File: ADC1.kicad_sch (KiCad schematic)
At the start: 21 parts, among them U8 MCP6004

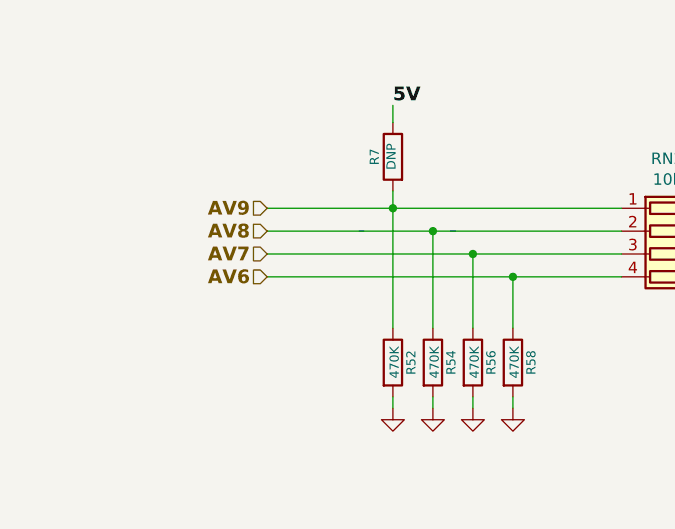
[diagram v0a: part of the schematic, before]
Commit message: haciendo el pcb
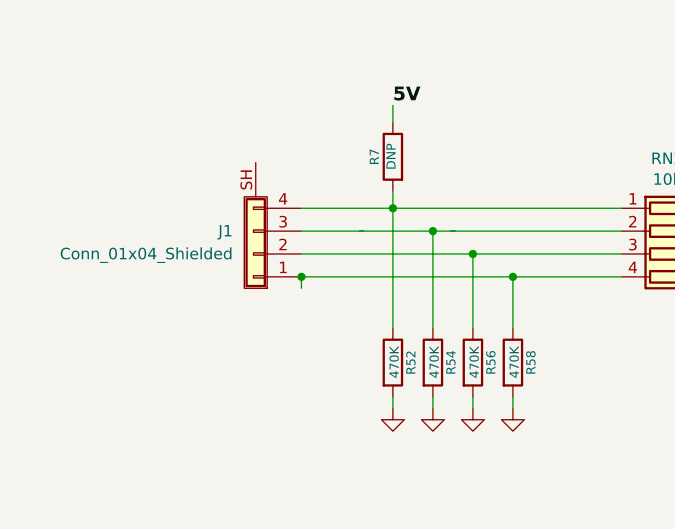
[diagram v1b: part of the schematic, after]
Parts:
- added J1: Conn_01x04_Shielded, Connector_Phoenix_SPT:PhoenixContact_SPT_2.5_4-H-5.0-EX_1x04_P5.0mm_Horizontal, symbol Connector_Generic_Shielded:Conn_01x04_Shielded
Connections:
- net AV6: no longer names the net of R58.1, RN2.4 (R4.1)
- net AV6: now also J1.1 (Pin_1)
- net AV7: no longer names the net of R56.1, RN2.3 (R3.1)
- net AV7: now also J1.2 (Pin_2)
- net AV8: no longer names the net of R54.1, RN2.2 (R2.1)
- net AV8: now also J1.3 (Pin_3)
- net AV9: no longer names the net of R52.1, R7.2, RN2.1 (R1.1)
- net AV9: now also J1.4 (Pin_4)
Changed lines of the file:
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@@
 	)
 	(junction
-		(at 191.77 66.04)
+		(at 87.63 85.09)
 		(diameter 0)
 		(color 0 0 0 0)
 	)
 	(junction
-		(at 87.63 85.09)
+		(at 68.58 87.63)
+		(diameter 0)
+		(color 0 0 0 0)
+	)
+	(junction
+		(at 191.77 66.04)
 		(diameter 0)
 		(color 0 0 0 0)
@@
 	)
 	(junction
-		(at 83.185 82.55)
+		(at 201.93 111.76)
 		(diameter 0)
 		(color 0 0 0 0)
 	)
 	(junction
-		(at 201.93 111.76)
+		(at 78.74 80.01)
 		(diameter 0)
 		(color 0 0 0 0)
 	)
 	(junction
-		(at 78.74 80.01)
+		(at 83.185 82.55)
 		(diameter 0)
 		(color 0 0 0 0)
@@
 	(wire
 		(pts
-			(xy 201.93 130.81) (xy 201.93 132.08)
+			(xy 68.58 85.09) (xy 87.63 85.09)
 		)
 		(stroke
@@
 	(wire
 		(pts
-			(xy 162.56 114.3) (xy 162.56 85.09)
-		)
-		(stroke
-			(width 0)
-			(type default)
-		)
-	)
-	(wire
-		(pts
-			(xy 142.24 109.855) (xy 142.24 80.01)
+			(xy 201.93 130.81) (xy 201.93 132.08)
 		)
 		(stroke
@@
 	(wire
 		(pts
-			(xy 64.77 87.63) (xy 92.075 87.63)
+			(xy 162.56 114.3) (xy 162.56 85.09)
 		)
 		(stroke
@@
 	(wire
 		(pts
-			(xy 83.185 82.55) (xy 104.14 82.55)
+			(xy 142.24 109.855) (xy 142.24 80.01)
 		)
 		(stroke
@@
 	(wire
 		(pts
-			(xy 92.075 87.63) (xy 104.14 87.63)
+			(xy 68.58 87.63) (xy 92.075 87.63)
 		)
 		(stroke
@@
 	(wire
 		(pts
-			(xy 64.77 80.01) (xy 78.74 80.01)
+			(xy 125.73 87.63) (xy 165.1 87.63)
 		)
 		(stroke
@@
 	(wire
 		(pts
-			(xy 87.63 93.345) (xy 87.63 85.09)
+			(xy 83.185 93.345) (xy 83.185 82.55)
 		)
 		(stroke
@@
 	(wire
 		(pts
-			(xy 125.73 87.63) (xy 165.1 87.63)
+			(xy 123.825 85.09) (xy 162.56 85.09)
 		)
 		(stroke
@@
 	(wire
 		(pts
-			(xy 83.185 93.345) (xy 83.185 82.55)
+			(xy 139.065 109.855) (xy 142.24 109.855)
 		)
 		(stroke
@@
 		)
 	)
-	(wire
+	(polyline
 		(pts
-			(xy 123.825 85.09) (xy 162.56 85.09)
+			(xy 74.93 82.55) (xy 75.565 82.55)
 		)
 		(stroke
 			(width 0)
-			(type default)
+			(type dash)
 		)
 	)
 	(wire
 		(pts
-			(xy 139.065 109.855) (xy 142.24 109.855)
+			(xy 78.74 68.58) (xy 78.74 70.485)
 		)
 		(stroke
@@
 		)
 	)
-	(polyline
+	(wire
 		(pts
-			(xy 74.93 82.55) (xy 75.565 82.55)
+			(xy 83.185 82.55) (xy 104.14 82.55)
 		)
 		(stroke
 			(width 0)
-			(type dash)
+			(type default)
 		)
 	)
 	(wire
 		(pts
-			(xy 78.74 68.58) (xy 78.74 70.485)
+			(xy 114.3 85.09) (xy 123.825 85.09)
 		)
 		(stroke
@@
 	(wire
 		(pts
-			(xy 114.3 85.09) (xy 123.825 85.09)
+			(xy 157.48 80.01) (xy 168.91 80.01)
 		)
 		(stroke
@@
 	(wire
 		(pts
-			(xy 157.48 80.01) (xy 168.91 80.01)
+			(xy 127 112.395) (xy 128.905 112.395)
 		)
 		(stroke
@@
 	(wire
 		(pts
-			(xy 127 112.395) (xy 128.905 112.395)
+			(xy 92.075 87.63) (xy 104.14 87.63)
 		)
 		(stroke
@@
 	(wire
 		(pts
+			(xy 68.58 82.55) (xy 83.185 82.55)
+		)
+		(stroke
+			(width 0)
+			(type default)
+		)
+	)
+	(wire
+		(pts
 			(xy 198.12 74.295) (xy 199.39 74.295)
 		)
@@
 	(wire
 		(pts
-			(xy 78.74 93.345) (xy 78.74 80.01)
+			(xy 78.74 80.01) (xy 78.74 93.345)
 		)
 		(stroke
@@
 		)
 	)
-	(wire
+	(polyline
 		(pts
-			(xy 64.77 82.55) (xy 83.185 82.55)
+			(xy 207.01 86.36) (xy 199.39 86.36)
 		)
 		(stroke
 			(width 0)
-			(type default)
+			(type dash)
 		)
 	)
 	(wire
 		(pts
-			(xy 64.77 85.09) (xy 87.63 85.09)
+			(xy 87.63 85.09) (xy 87.63 93.345)
 		)
 		(stroke
@@
 		)
 	)
-	(polyline
+	(wire
 		(pts
-			(xy 207.01 86.36) (xy 199.39 86.36)
+			(xy 217.17 87.63) (xy 219.71 87.63)
 		)
 		(stroke
 			(width 0)
-			(type dash)
+			(type default)
 		)
 	)
 	(wire
 		(pts
-			(xy 217.17 87.63) (xy 219.71 87.63)
+			(xy 144.145 114.935) (xy 144.145 82.55)
 		)
 		(stroke
@@
 	(wire
 		(pts
-			(xy 144.145 114.935) (xy 144.145 82.55)
+			(xy 78.74 80.01) (xy 104.14 80.01)
 		)
 		(stroke
@@
 	(wire
 		(pts
-			(xy 78.74 80.01) (xy 104.14 80.01)
+			(xy 176.53 76.2) (xy 172.72 76.2)
 		)
 		(stroke
@@
 	(wire
 		(pts
-			(xy 176.53 76.2) (xy 172.72 76.2)
+			(xy 68.58 88.9) (xy 68.58 87.63)
 		)
 		(stroke
@@
 	(wire
 		(pts
+			(xy 68.58 80.01) (xy 78.74 80.01)
+		)
+		(stroke
+			(width 0)
+			(type default)
+		)
+	)
+	(wire
+		(pts
 			(xy 191.77 104.14) (xy 198.12 104.14)
 		)
@@
 		)
 	)
-	(hierarchical_label "AV8"
-		(shape input)
-		(at 64.77 82.55 180)
-		(effects
-			(font
-				(size 1.524 1.524)
-				(thickness 0.3048)
-				(bold yes)
-			)
-			(justify right)
-		)
-	)
-	(hierarchical_label "AV6"
-		(shape input)
-		(at 64.77 87.63 180)
-		(effects
-			(font
-				(size 1.524 1.524)
-				(thickness 0.3048)
-				(bold yes)
-			)
-			(justify right)
-		)
-	)
 	(hierarchical_label "AV6_MCU"
 		(shape input)
@@
 		)
 	)
-	(hierarchical_label "AV9"
-		(shape input)
-		(at 64.77 80.01 180)
-		(effects
-			(font
-				(size 1.524 1.524)
-				(thickness 0.3048)
-				(bold yes)
-			)
-			(justify right)
-		)
-	)
 	(hierarchical_label "AV8_MCU"
 		(shape input)
@@
 		)
 	)
-	(hierarchical_label "AV7"
-		(shape input)
-		(at 64.77 85.09 180)
-		(effects
-			(font
-				(size 1.524 1.524)
-				(thickness 0.3048)
-				(bold yes)
-			)
-			(justify right)
-		)
-	)
 	(symbol
 		(lib_id "Device:C")
@@
 					(unit 1)
 				)
+			)
+		)
+	)
+	(symbol
+		(lib_id "Connector_Generic_Shielded:Conn_01x04_Shielded")
+		(at 63.5 85.09 180)
+		(unit 1)
+		(body_style 1)
+		(exclude_from_sim no)
+		(in_bom yes)
+		(on_board yes)
+		(in_pos_files yes)
+		(dnp no)
+		(fields_autoplaced yes)
+		(property "Reference" "J1"
+			(at 60.96 82.5499 0)
+			(show_name no)
+			(do_not_autoplace no)
+			(effects
+				(font
+					(size 1.27 1.27)
+				)
+				(justify left)
+			)
+		)
+		(property "Value" "Conn_01x04_Shielded"
+			(at 60.96 85.0899 0)
+			(show_name no)
+			(do_not_autoplace no)
+			(effects
+				(font
+					(size 1.27 1.27)
+				)
+				(justify left)
+			)
+		)
+		(property "Footprint" "Connector_Phoenix_SPT:PhoenixContact_SPT_2.5_4-H-5.0-EX_1x04_P5.0mm_Horizontal"
+			(at 63.5 85.09 0)
+			(hide yes)
+			(show_name no)
+			(do_not_autoplace no)
+			(effects
+				(font
+					(size 1.27 1.27)
+				)
+			)
+		)
+		(property "Datasheet" ""
+			(at 63.5 85.09 0)
+			(hide yes)
+			(show_name no)
+			(do_not_autoplace no)
+			(effects
+				(font
+					(size 1.27 1.27)
+				)
+			)
+		)
+		(property "Description" "Generic shielded connector, single row, 01x04, script generated (kicad-library-utils/schlib/autogen/connector/)"
+			(at 63.5 85.09 0)
+			(hide yes)
+			(show_name no)
+			(do_not_autoplace no)
+			(effects
+				(font
+					(size 1.27 1.27)
+				)
+			)
+		)
+		(pin "SH"
+		)
+		(pin "4"
+		)
+		(pin "1"
+		)
+		(pin "2"
+		)
+		(pin "3"
+		)
+		(instances
+			(project "ADC1"
+				(path "/2a1381e6-d7f3-4ca8-8ebb-da5f70281df7"
+					(reference "J1")
+					(unit 1)
+				)
